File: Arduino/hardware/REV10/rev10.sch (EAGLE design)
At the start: 26 parts, among them IC2 ATMEGA168-AU, Q1 32768Hz, U1 TC1185SMD, U2 ARDUINOR3-DIMENSION

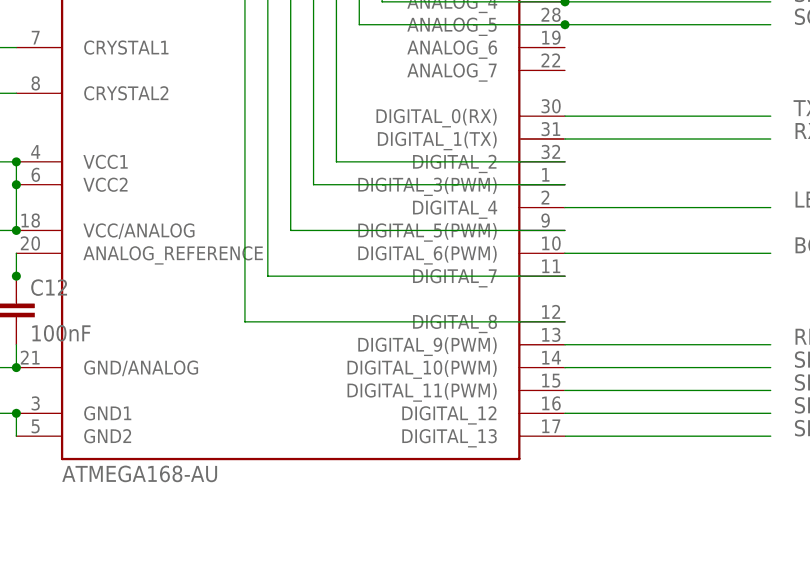
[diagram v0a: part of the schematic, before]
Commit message: updates to rev10 as per deniz spec
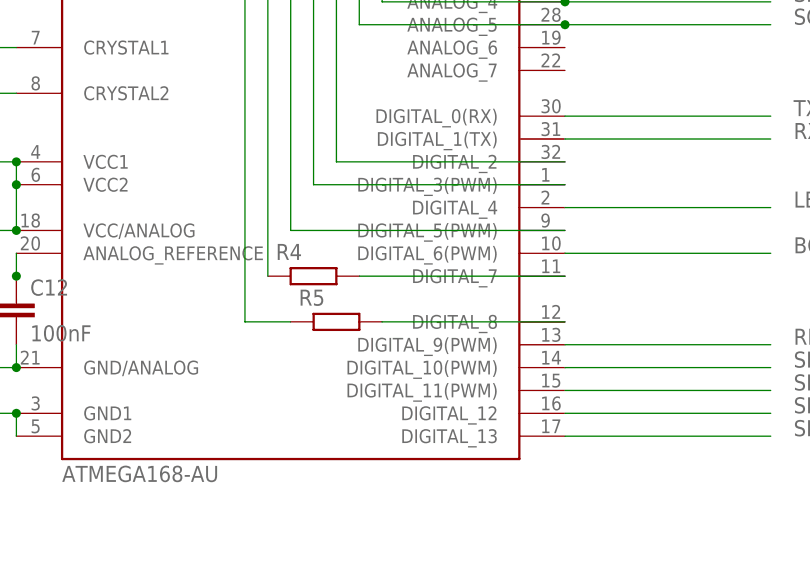
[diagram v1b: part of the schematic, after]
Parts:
- added R4: 4.7K, resistor:R-EU_R0603
- added R5: 330R, resistor:R-EU_R0603
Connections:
- new net N$1: IC2.DIGITAL_7, R4.1
- new net N$3: IC2.DIGITAL_8, R5.1
- net N$19: now also R5.2; no longer IC2.DIGITAL_8
- net N$21: now also R4.2; no longer IC2.DIGITAL_7
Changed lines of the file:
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@@
 <?xml version="1.0" encoding="utf-8"?>
 <!DOCTYPE eagle SYSTEM "eagle.dtd">
-<eagle version="7.3.0">
+<eagle version="7.4.0">
 <drawing>
 <settings>
@@
 <part name="I2C_EXT" library="pinhead" deviceset="PINHD-2X7" device=""/>
 <part name="IC2" library="Arduino-AVR" deviceset="ATMEGA168" device="-AU"/>
+<part name="R4" library="resistor" deviceset="R-EU_" device="R0603" value="4.7K"/>
+<part name="R5" library="resistor" deviceset="R-EU_" device="R0603" value="330R"/>
 </parts>
 <sheets>
@@
 <instance part="I2C_EXT" gate="A" x="124.46" y="213.36" rot="R90"/>
 <instance part="IC2" gate="1" x="195.58" y="91.44"/>
+<instance part="R4" gate="G$1" x="198.12" y="78.74" smashed="yes" rot="R180">
+<attribute name="NAME" x="196.85" y="82.3214" size="1.778" layer="95" rot="R180"/>
+</instance>
+<instance part="R5" gate="G$1" x="200.66" y="73.66" smashed="yes" rot="R180">
+<attribute name="NAME" x="199.39" y="77.2414" size="1.778" layer="95" rot="R180"/>
+</instance>
 </instances>
 <busses>
@@
 <net name="N$21" class="0">
 <segment>
-<wire x1="226.06" y1="78.74" x2="193.04" y2="78.74" width="0.1524" layer="91"/>
 <wire x1="193.04" y1="78.74" x2="193.04" y2="162.56" width="0.1524" layer="91"/>
 <wire x1="193.04" y1="162.56" x2="167.64" y2="162.56" width="0.1524" layer="91"/>
-<pinref part="IC2" gate="1" pin="DIGITAL_7"/>
+<pinref part="R4" gate="G$1" pin="2"/>
 </segment>
 </net>
 <net name="N$19" class="0">
 <segment>
-<wire x1="226.06" y1="73.66" x2="190.5" y2="73.66" width="0.1524" layer="91"/>
 <wire x1="190.5" y1="73.66" x2="190.5" y2="157.48" width="0.1524" layer="91"/>
 <pinref part="U2" gate="G$1" pin="D8"/>
 <wire x1="190.5" y1="157.48" x2="167.64" y2="157.48" width="0.1524" layer="91"/>
-<pinref part="IC2" gate="1" pin="DIGITAL_8"/>
+<pinref part="R5" gate="G$1" pin="2"/>
+<wire x1="195.58" y1="73.66" x2="190.5" y2="73.66" width="0.1524" layer="91"/>
 </segment>
 </net>
@@
 </segment>
 </net>
+<net name="N$1" class="0">
+<segment>
+<pinref part="R4" gate="G$1" pin="1"/>
+<pinref part="IC2" gate="1" pin="DIGITAL_7"/>
+<wire x1="203.2" y1="78.74" x2="226.06" y2="78.74" width="0.1524" layer="91"/>
+</segment>
+</net>
+<net name="N$3" class="0">
+<segment>
+<pinref part="R5" gate="G$1" pin="1"/>
+<pinref part="IC2" gate="1" pin="DIGITAL_8"/>
+<wire x1="205.74" y1="73.66" x2="226.06" y2="73.66" width="0.1524" layer="91"/>
+</segment>
+</net>

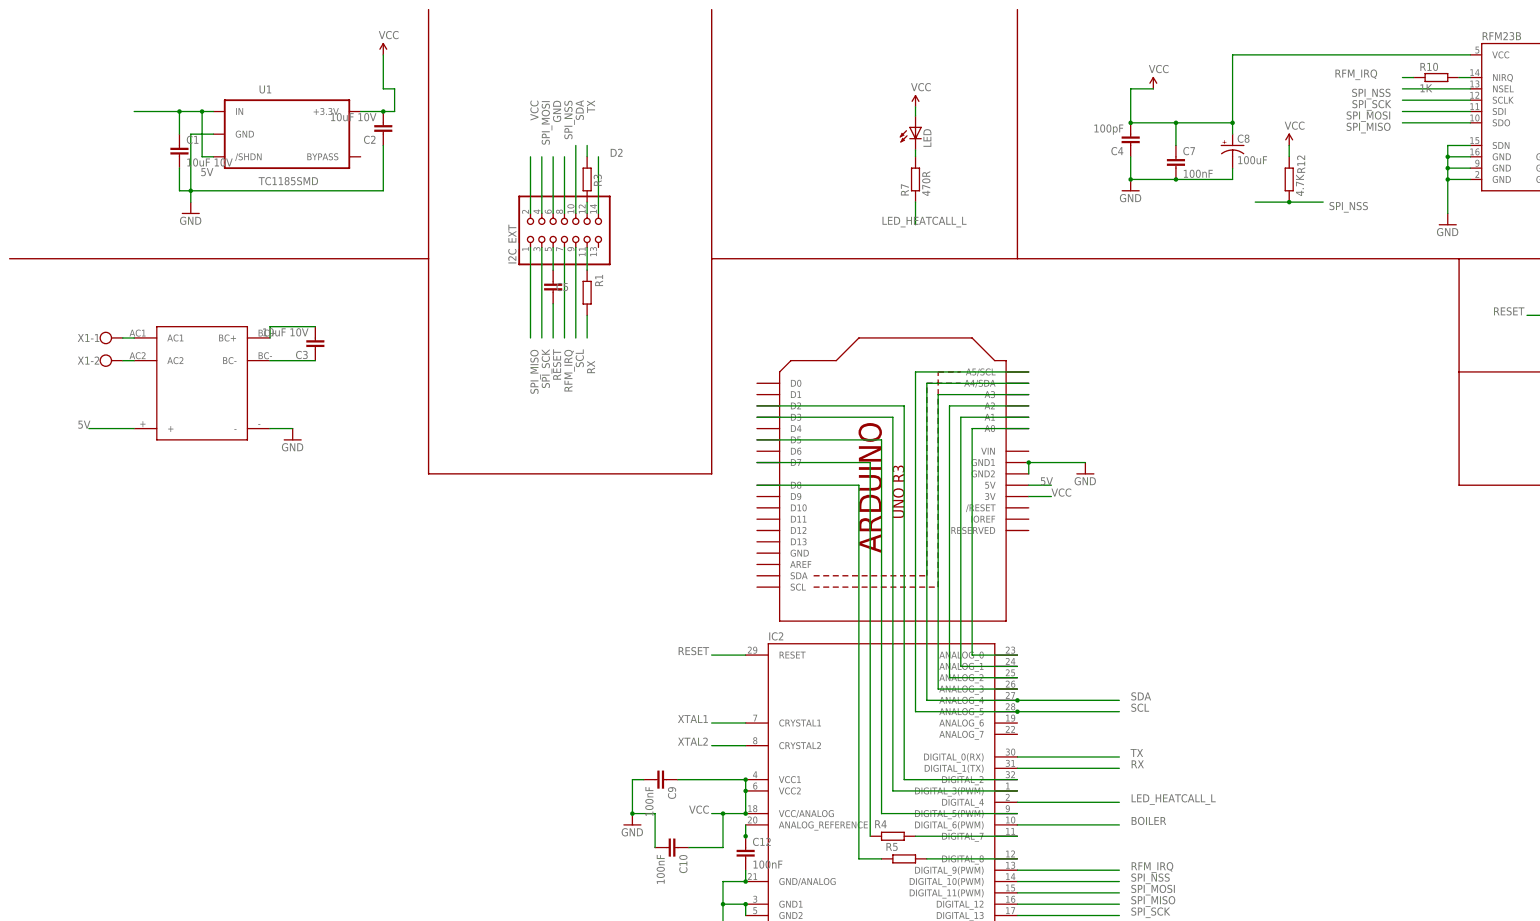
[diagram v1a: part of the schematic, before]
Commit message: updates as pr google doc
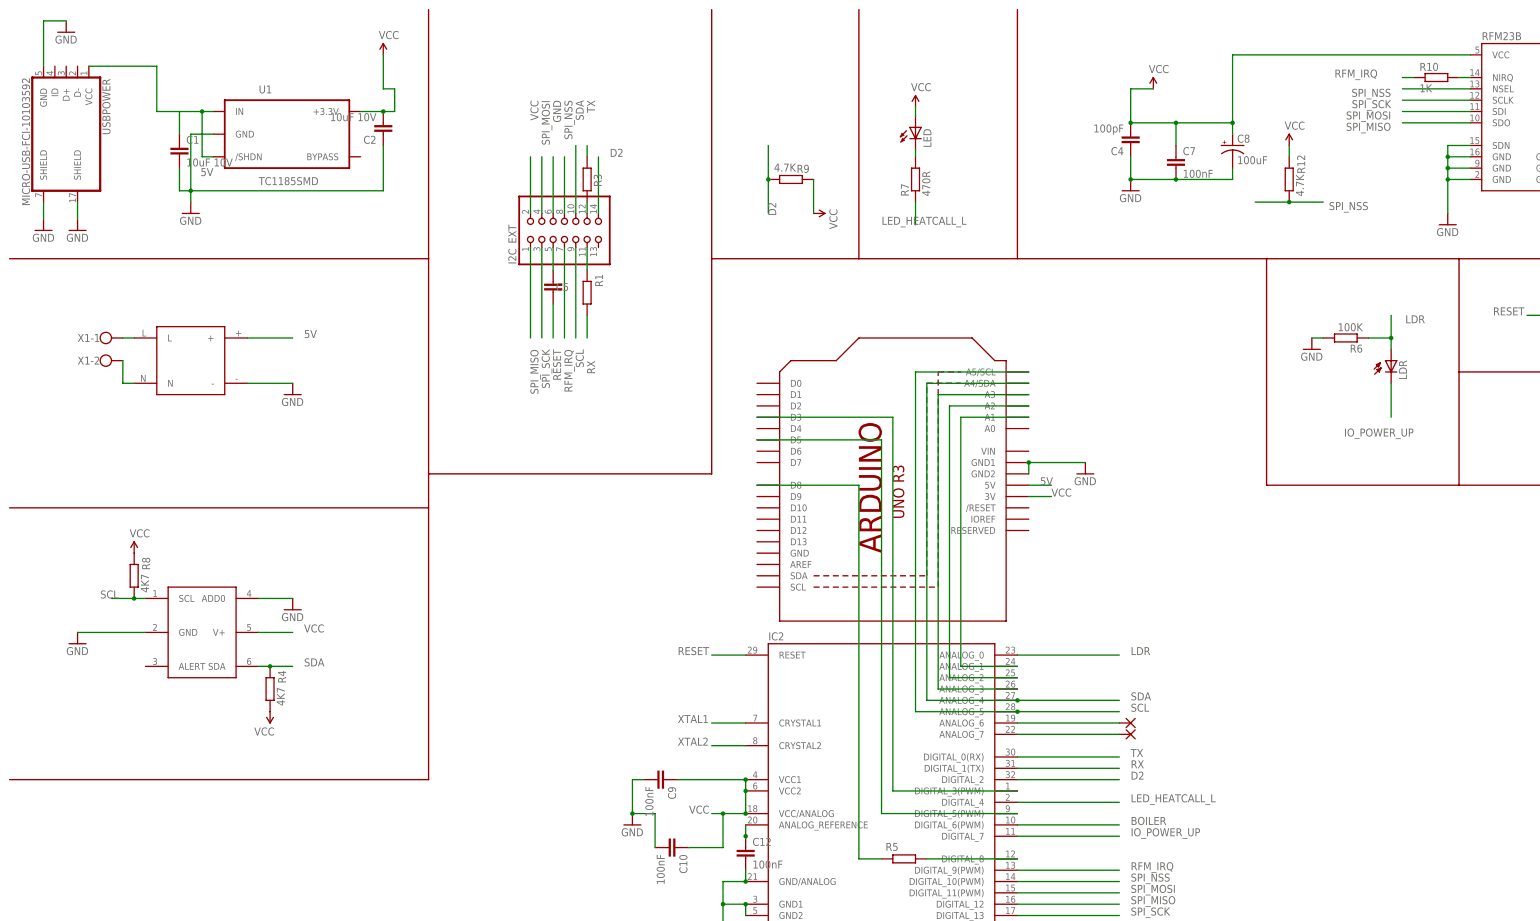
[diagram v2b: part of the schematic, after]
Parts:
- removed C3: 10uF 10V, resistor:C-EUC0603
- removed U$3: TUHS10, tuhs10:TUHS10
- added A6, A7: WIREPAD1,6/0,9, wirepad:WIREPAD1,6/0,9
- added LDR: BPX65, opto-trans-siemens:BPX65
- added R6: 100K, resistor:R-EU_R0603
- added R8: 4K7, resistor:R-EU_R0603
- added R9: 4.7K, resistor:R-EU_R0603
- added TMP112: TMP1, TMP112_2:TMP112
- added U$4: VTX-214-010-205, VTX-214-010-205:VTX-214-010-205
- added USBPOWER: MICRO-USB-FCI-10103592, micro-usb-fci-10103592:MICRO-USB-FCI-10103592
- I2C_EXT: device pinhead:PINHD-2X7 -> pinhead:PINHD-2X7/90
- R4: value 4.7K -> 4K7
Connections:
- removed net N$11: C3.1, U$3.BC-
- removed net N$12: C3.2, U$3.BC+
- removed net N$14: IC2.ANALOG_0, U2.A0
- removed net N$21: R4.2
- removed net N$22: IC2.DIGITAL_2, U2.D2
- new net 5V1: USBPOWER.VCC
- new net IO_POWER_UP: IC2.DIGITAL_7, LDR.C
- new net LDR: IC2.ANALOG_0, LDR.A, R6.1
- new net N$5: A7.P, IC2.ANALOG_7
- net 5V: no longer U$3.+
- net D2: now also IC2.DIGITAL_2, R9.1
- net GND: now also R6.2, TMP112.ADD0, TMP112.GND, USBPOWER.GND, USBPOWER.SHIELD@5, USBPOWER.SHIELD@8; no longer U$3.-
- net N$1: now also A6.P, IC2.ANALOG_6; no longer IC2.DIGITAL_7, R4.1
- net N$4: no longer U$3.AC2
- net N$8: now also U$4.L; no longer U$3.AC1
- net SCL: now also R8.1, TMP112.SCL
- net SDA: now also R4.2, TMP112.SDA
- net VCC: now also R4.1, R8.2, R9.2, TMP112.V+
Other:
- moved on the sheet: R4

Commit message: updates as pr google doc and guidance from mark and deniz
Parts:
- removed A6, A7: WIREPAD1,6/0,9, wirepad:WIREPAD1,6/0,9
- added JP1: (no value), pinhead:PINHD-2X4/90
- added LED1: (no value), adafruit:LED3MM
- added R11: 470R, resistor:R-EU_R0603
- added R13: 1K, resistor:R-EU_R0603
- added R14: 10K, resistor:R-EU_R0603
- added T1: (no value), transistor:-NPN-SOT23-EBC
- added X2: (no value), con-wago-500:W237-102
- renumbered LDR to PHT, U$4 to PSU
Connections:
- removed net N$17: IC2.ANALOG_3, U2.A3
- removed net N$24: IC2.DIGITAL_3(PWM), U2.D3
- new net N$11: IC2.ANALOG_2
- new net N$12: R13.2, R14.2, T1.B
- new net N$14: LED1.C, T1.C, X2-1.KL
- new net VOICE: IC2.DIGITAL_3(PWM)
- net 5V: now also R11.2, X2-2.KL
- net BOILER: now also R13.1
- net GND: now also JP1.5, R14.1, T1.E, U2.GND
- net N$1: now also JP1.1; no longer A6.P
- net N$16: now also LED1.A, R11.1; no longer IC2.ANALOG_2, U2.A2
- net N$19: no longer U2.D8
- net N$20: no longer U2.D5
- net N$5: now also JP1.3; no longer A7.P
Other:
- note added: "On BOM"
